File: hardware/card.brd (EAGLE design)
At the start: 97 x 56 mm, 93 parts, among them J1 UE27AC54100, J2 MICROSD, J3 0541323062, J4 6-PIN_2MM-V, J5 JST_2PIN, J6 B2PS-VH(LF)(SN), J7 MINI-USB-UX60A-MB-5ST, J8 JST_2PIN, U1 ATSAMD21J_QFN, U2 TS3USB221, U3 MIC2288YD5-TR, U4 MCP73833, U5 TLV70233DBVR, X2 32.768, X3 ATWINC1500_MR210PA

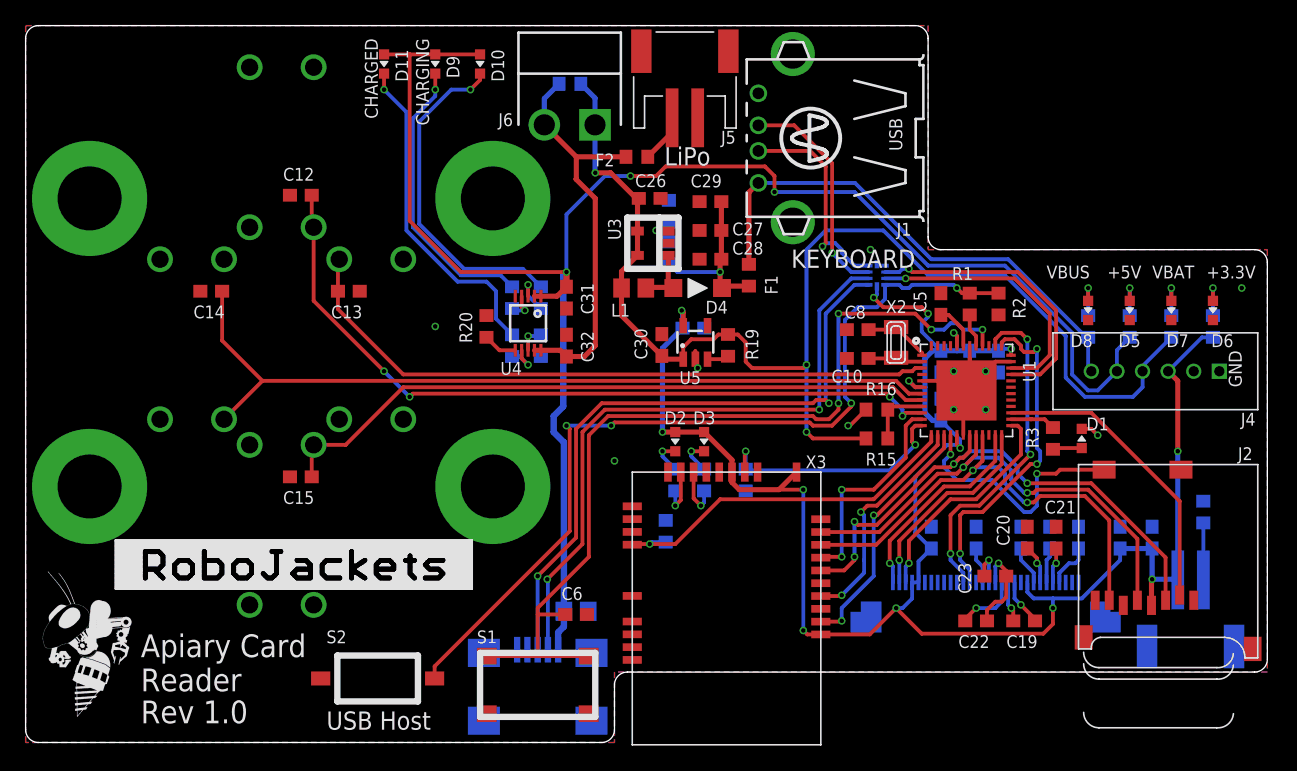
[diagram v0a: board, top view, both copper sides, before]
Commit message: More tweaks, fix DRC error
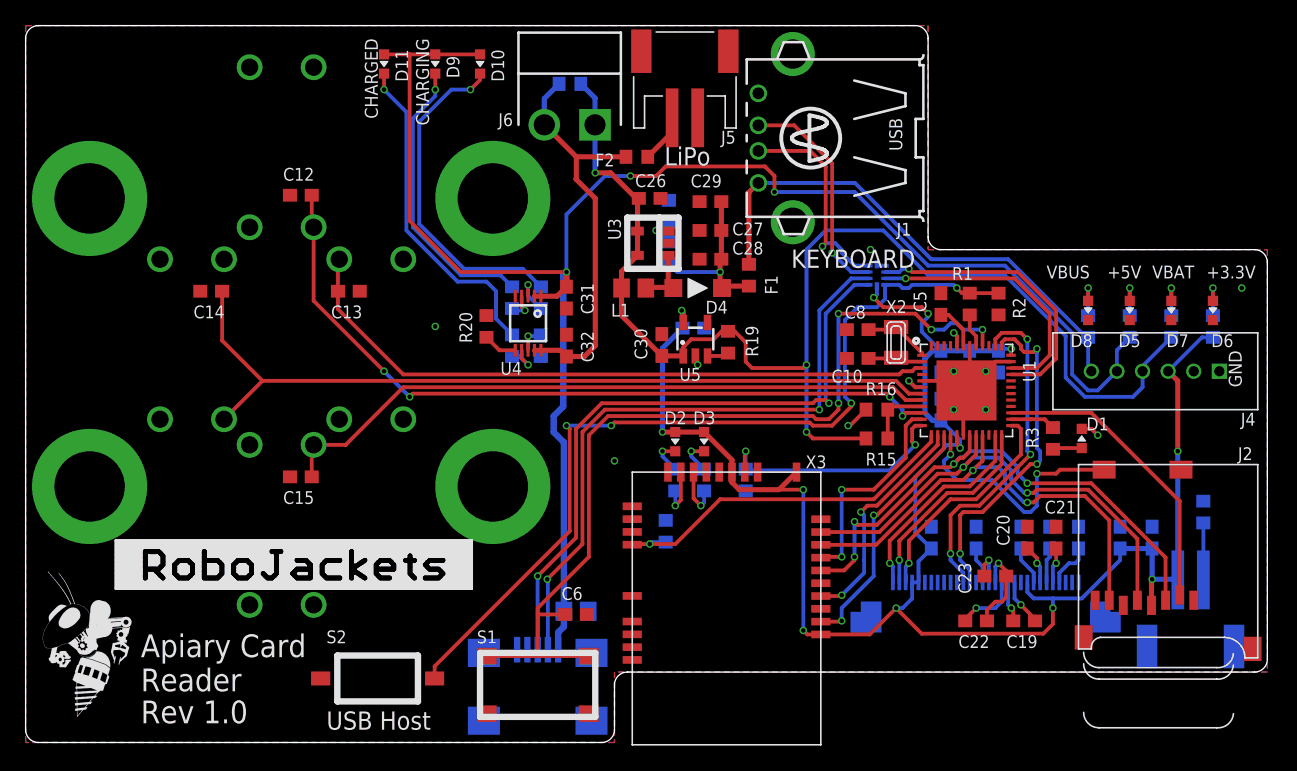
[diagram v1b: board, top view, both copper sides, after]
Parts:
- moved R19 0.25 mm to (54.9, 31.3)
- moved U5 0.25 mm to (52.3, 31.5)
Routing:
- net GND: track 16.9 -> 15.8 mm
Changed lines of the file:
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@@
 <text x="42" y="51" size="1.016" layer="22" rot="MR180">np</text>
 <text x="60" y="11" size="1.4224" layer="22" font="vector" rot="MR180">LCD</text>
-<text x="96.5" y="15.5" size="1.4224" layer="22" font="vector" rot="MR0">LCD</text>
+<text x="95.75" y="15.5" size="1.4224" layer="22" font="vector" rot="MR0">LCD</text>
 <text x="30.5" y="55" size="1.016" layer="21" font="vector" rot="R270">CHARGING</text>
 <text x="26.5" y="55" size="1.016" layer="21" font="vector" rot="R270">CHARGED</text>
@@
 </class>
 </classes>
-<designrules name="eC_2Layer_PClass6_BaseCopperO18_eCDefault *">
+<designrules name="eC_2Layer_PClass6_BaseCopperO18_eCDefault">
 <description language="de">
 &lt;p&gt;
@@
 <param name="srMaxRoundness" value="0mil"/>
 <param name="slThermalIsolate" value="0.2mm"/>
-<param name="slThermalsForVias" value="0"/>
+<param name="slThermalsForVias" value="1"/>
 <param name="dpMaxLengthDifference" value="10mm"/>
 <param name="dpGapFactor" value="2.5"/>
@@
 </element>
 <element name="R4" library="rcl" library_urn="urn:adsk.eagle:library:334" package="R0603" package3d_urn="urn:adsk.eagle:package:23555/2" value="0" x="92" y="18" smashed="yes" rot="MR90">
-<attribute name="NAME" x="93.135" y="17.115" size="1" layer="26" rot="MR90"/>
+<attribute name="NAME" x="92.885" y="17.865" size="1" layer="26" rot="MR90"/>
 <attribute name="VALUE" x="90.095" y="17.365" size="1.27" layer="28" rot="MR90"/>
 </element>
@@
 <attribute name="VALUE" x="65.865" y="21.845" size="1.27" layer="27"/>
 </element>
-<element name="R19" library="rcl" library_urn="urn:adsk.eagle:library:334" package="R0603" package3d_urn="urn:adsk.eagle:package:23555/2" value="10k" x="54.87" y="31.02" smashed="yes" rot="R90">
-<attribute name="NAME" x="57.235" y="29.885" size="1" layer="25" rot="R90"/>
-<attribute name="VALUE" x="56.775" y="30.385" size="1.27" layer="27" rot="R90"/>
+<element name="R19" library="rcl" library_urn="urn:adsk.eagle:library:334" package="R0603" package3d_urn="urn:adsk.eagle:package:23555/2" value="10k" x="54.87" y="31.27" smashed="yes" rot="R90">
+<attribute name="NAME" x="57.235" y="30.135" size="1" layer="25" rot="R90"/>
+<attribute name="VALUE" x="56.775" y="30.635" size="1.27" layer="27" rot="R90"/>
 </element>
 <element name="R16" library="rcl" library_urn="urn:adsk.eagle:library:334" package="R0603" package3d_urn="urn:adsk.eagle:package:23555/2" value="10k 1%" x="66.5" y="26" smashed="yes" rot="R180">
@@
 <attribute name="VALUE" x="36.968" y="34.274" size="0.5" layer="27" ratio="10" rot="R270"/>
 </element>
-<element name="U5" library="lib-card" package="SOT-23-5" value="TLV70233DBVR" x="52.32" y="31.25" smashed="yes">
-<attribute name="DIGIKEY" value="296-32415-1-ND" x="52.32" y="31.25" size="1.778" layer="27" display="off"/>
-<attribute name="MPN" value="TLV70233DBVR" x="52.32" y="31.25" size="1.778" layer="27" display="off"/>
-<attribute name="NAME" x="51.07" y="28" size="1" layer="25" ratio="10"/>
+<element name="U5" library="lib-card" package="SOT-23-5" value="TLV70233DBVR" x="52.32" y="31.5" smashed="yes">
+<attribute name="DIGIKEY" value="296-32415-1-ND" x="52.32" y="31.5" size="1.778" layer="27" display="off"/>
+<attribute name="MPN" value="TLV70233DBVR" x="52.32" y="31.5" size="1.778" layer="27" display="off"/>
+<attribute name="NAME" x="51.07" y="28.25" size="1" layer="25" ratio="10"/>
 </element>
 <element name="X3" library="CardReader" package="ATWINC1500_MR210PA" value="ATWINC1500_MR210PA" x="54.5" y="13.5" smashed="yes" rot="R180">
@@
 <wire x1="76.975" y1="29.75" x2="75.75" y2="29.75" width="0.3" layer="1"/>
 <wire x1="75.75" y1="29.75" x2="75.5" y2="29.5" width="0.3" layer="1"/>
-<wire x1="73.75" y1="30.975" x2="73.75" y2="30" width="0.3" layer="1"/>
-<wire x1="73.75" y1="30" x2="73.75" y2="29.75" width="0.3" layer="1"/>
+<wire x1="73.75" y1="30.975" x2="73.75" y2="29.75" width="0.3" layer="1"/>
 <wire x1="73.5" y1="29.5" x2="73.75" y2="29.75" width="0.3" layer="1"/>
 <polygon width="0.3" layer="16">
@@
 <wire x1="73.5" y1="27.5" x2="73.5" y2="26" width="0.3" layer="1"/>
 <wire x1="73.5" y1="26" x2="72.5" y2="26" width="0.3" layer="1"/>
-<wire x1="73.75" y1="30" x2="73.75" y2="27.5" width="0.3" layer="1"/>
+<wire x1="73.75" y1="29.75" x2="73.75" y2="27.5" width="0.3" layer="1"/>
 <wire x1="73.75" y1="27.5" x2="73.5" y2="27.5" width="0.3" layer="1"/>
-<wire x1="52.32" y1="29.944" x2="52.32" y2="30.57" width="0.3" layer="1"/>
-<wire x1="52.32" y1="30.57" x2="52.5" y2="29.25" width="0.3" layer="1"/>
-<via x="52.5" y="29.25" extent="1-16" drill="0.35"/>
+<wire x1="52.32" y1="30.57" x2="52.32" y2="30.194" width="0.3" layer="1"/>
+<via x="52.5" y="29.5" extent="1-16" drill="0.35"/>
 <wire x1="65.65" y1="26" x2="64.4" y2="24.75" width="0.3" layer="1"/>
 <wire x1="64.4" y1="24.75" x2="64.25" y2="24.75" width="0.3" layer="1"/>
@@
 <contactref element="S4" pad="4"/>
 <contactref element="S3" pad="4"/>
+<wire x1="52.32" y1="30.194" x2="52.32" y2="29.68" width="0.3" layer="1"/>
+<wire x1="52.32" y1="29.68" x2="52.5" y2="29.5" width="0.3" layer="1"/>
 </signal>
 <signal name="D-">
@@
 <via x="51.25" y="33.75" extent="1-16" drill="0.35"/>
 <wire x1="51.25" y1="33.75" x2="51.37" y2="33.63" width="0.4" layer="1"/>
-<wire x1="51.37" y1="33.63" x2="51.37" y2="32.556" width="0.4" layer="1"/>
+<wire x1="51.37" y1="33.63" x2="51.37" y2="32.806" width="0.4" layer="1"/>
 <wire x1="71.5" y1="30.6" x2="70" y2="32.1" width="0.3" layer="16"/>
 <wire x1="70" y1="32.1" x2="70" y2="32.75" width="0.3" layer="16"/>
@@
 <wire x1="46.55" y1="33.35" x2="49.7" y2="30.2" width="0.4" layer="1"/>
 <wire x1="46.55" y1="33.35" x2="46.55" y2="35.5" width="0.4" layer="1"/>
-<wire x1="49.7" y1="30.2" x2="49.956" y2="29.944" width="0.4" layer="1"/>
-<wire x1="49.956" y1="29.944" x2="51.37" y2="29.944" width="0.4" layer="1"/>
+<wire x1="49.7" y1="30.2" x2="49.956" y2="30.194" width="0.4" layer="1"/>
+<wire x1="49.956" y1="30.194" x2="51.37" y2="30.194" width="0.4" layer="1"/>
 <wire x1="65.65" y1="23.75" x2="61.5" y2="23.75" width="0.3" layer="1"/>
 <wire x1="61.5" y1="23.75" x2="61" y2="24.25" width="0.3" layer="1"/>
@@
 <wire x1="56.75" y1="29.25" x2="56.25" y2="29.75" width="0.3" layer="1"/>
 <wire x1="56.25" y1="29.75" x2="56.25" y2="31.25" width="0.3" layer="1"/>
-<wire x1="56.25" y1="31.25" x2="55.63" y2="31.87" width="0.3" layer="1"/>
-<wire x1="55.63" y1="31.87" x2="54.87" y2="31.87" width="0.3" layer="1"/>
-<wire x1="54.87" y1="31.87" x2="54.12" y2="31.87" width="0.3" layer="1"/>
-<wire x1="54.12" y1="31.87" x2="53.75" y2="31.5" width="0.3" layer="1"/>
+<wire x1="56.25" y1="31.25" x2="55.38" y2="32.12" width="0.3" layer="1"/>
+<wire x1="55.38" y1="32.12" x2="54.87" y2="32.12" width="0.3" layer="1"/>
+<wire x1="54.87" y1="32.12" x2="54.37" y2="32.12" width="0.3" layer="1"/>
+<wire x1="54.37" y1="32.12" x2="53.75" y2="31.5" width="0.3" layer="1"/>
 <wire x1="52" y1="31.5" x2="53.75" y2="31.5" width="0.3" layer="1"/>
-<wire x1="51.37" y1="29.944" x2="51.37" y2="30.87" width="0.3" layer="1"/>
+<wire x1="51.37" y1="30.194" x2="51.37" y2="30.87" width="0.3" layer="1"/>
 <wire x1="51.37" y1="30.87" x2="52" y2="31.5" width="0.3" layer="1"/>
 <wire x1="61" y1="29.5" x2="61" y2="38.5" width="0.3" layer="16"/>
@@
 <contactref element="U5" pad="3"/>
 <contactref element="R19" pad="1"/>
-<wire x1="53.27" y1="29.944" x2="54.644" y2="29.944" width="0.3" layer="1"/>
-<wire x1="54.644" y1="29.944" x2="54.87" y2="30.17" width="0.3" layer="1"/>
+<wire x1="53.27" y1="30.194" x2="54.644" y2="30.194" width="0.3" layer="1"/>
+<wire x1="54.644" y1="30.194" x2="54.87" y2="30.42" width="0.3" layer="1"/>
 </signal>
 <signal name="BATT">
@@
 </signal>
 <signal name="N$1">
-<via x="36.5" y="42.5" extent="1-16" drill="5" diameter="9"/>
+<via x="36.5" y="42.5" extent="1-16" drill="5.5" diameter="9"/>
 </signal>
 <signal name="N$2">
-<via x="5" y="42.5" extent="1-16" drill="5" diameter="9"/>
+<via x="5" y="42.5" extent="1-16" drill="5.5" diameter="9"/>
 </signal>
 <signal name="N$3">
-<via x="5" y="20" extent="1-16" drill="5" diameter="9"/>
+<via x="5" y="20" extent="1-16" drill="5.5" diameter="9"/>
 </signal>
 <signal name="N$4">
-<via x="36.5" y="20" extent="1-16" drill="5" diameter="9"/>
+<via x="36.5" y="20" extent="1-16" drill="5.5" diameter="9"/>
 </signal>
 </signals>
